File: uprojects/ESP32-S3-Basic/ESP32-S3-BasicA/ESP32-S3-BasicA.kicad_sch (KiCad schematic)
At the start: 18 parts, among them J1 USB_C_Receptacle, Q1 BC817, Q2 BC817, SW1 ESP32_EN, SW2 ESP32_EN, U1 ESP32-S3-WROOM-1x-N8R8, U2 CH340G, Y1 12MHz

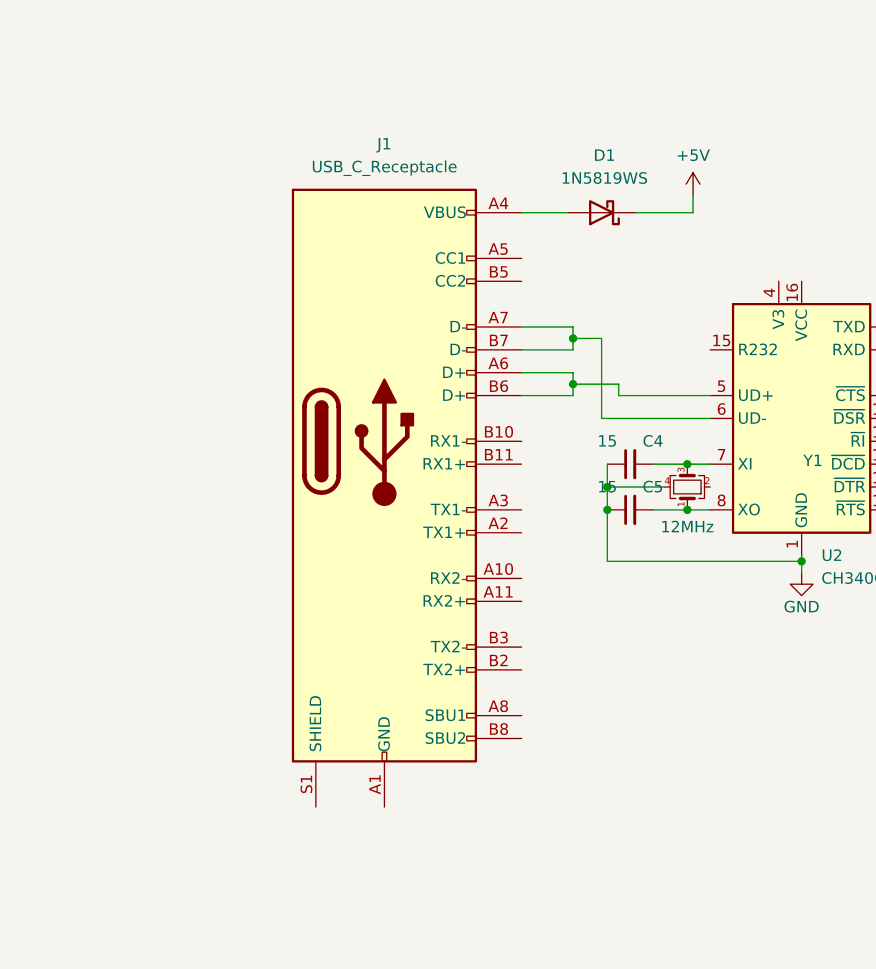
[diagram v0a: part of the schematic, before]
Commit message: April 3 commit
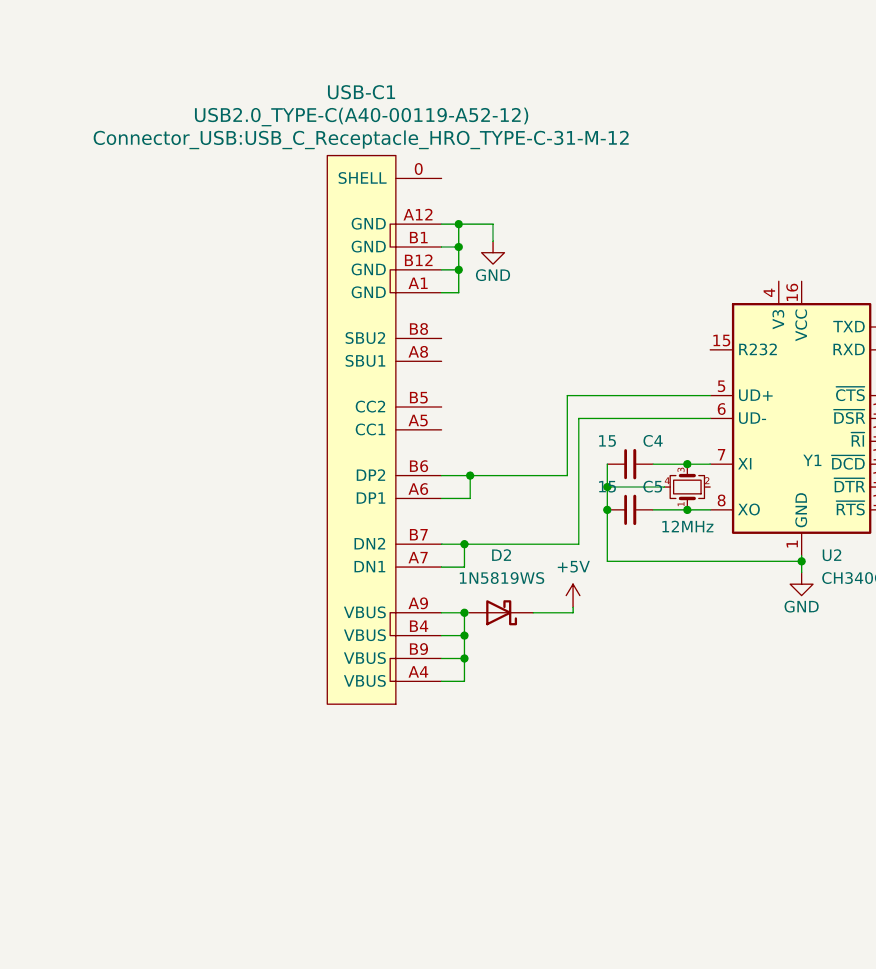
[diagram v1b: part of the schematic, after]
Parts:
- removed D1: 1N5819WS, Diode_SMD:D_SOD-323, symbol Diode:1N5819WS
- removed J1: USB_C_Receptacle, Connector_USB:USB_C_Receptacle_Amphenol_12401548E4-2A_CircularHoles, symbol Connector:USB_C_Receptacle
- added D2: 1N5819WS, Diode_SMD:D_SOD-323, symbol Diode:1N5819WS
- added USB-C1: USB2.0_TYPE-C(A40-00119-A52-12), Connector_USB:USB_C_Receptacle_HRO_TYPE-C-31-M-12, symbol ESP32-S3-DevKit-LiPo_Rev_B:USB2.0_TYPE-C(A40-00119-A52-12)
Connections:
- net +5V: now also D2.1 (K)
- net GND: now also USB-C1.A1 (GND), USB-C1.A12 (GND), USB-C1.B1 (GND), USB-C1.B12 (GND)
- net at U2.5 (UD+): now also USB-C1.A6 (DP1), USB-C1.B6 (DP2)
- net at U2.6 (UD-): now also USB-C1.A7 (DN1), USB-C1.B7 (DN2)
- new net: D2.2 (A), USB-C1.A4 (VBUS), USB-C1.A9 (VBUS), USB-C1.B4 (VBUS), USB-C1.B9 (VBUS)
